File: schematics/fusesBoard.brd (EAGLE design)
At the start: 25 parts, among them Q1 IRF540, Q2 IRF540, Q3 IRF540

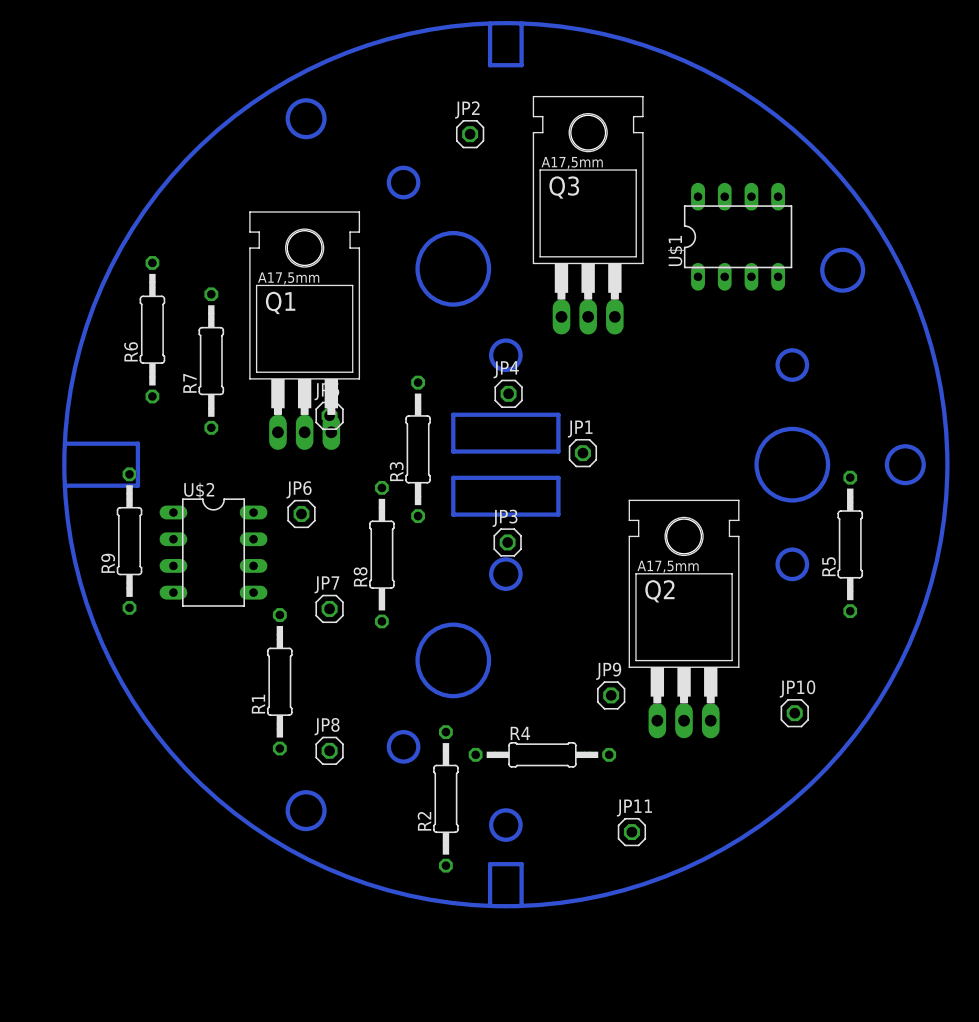
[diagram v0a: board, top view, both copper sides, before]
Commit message: разведена плата для пережигателей
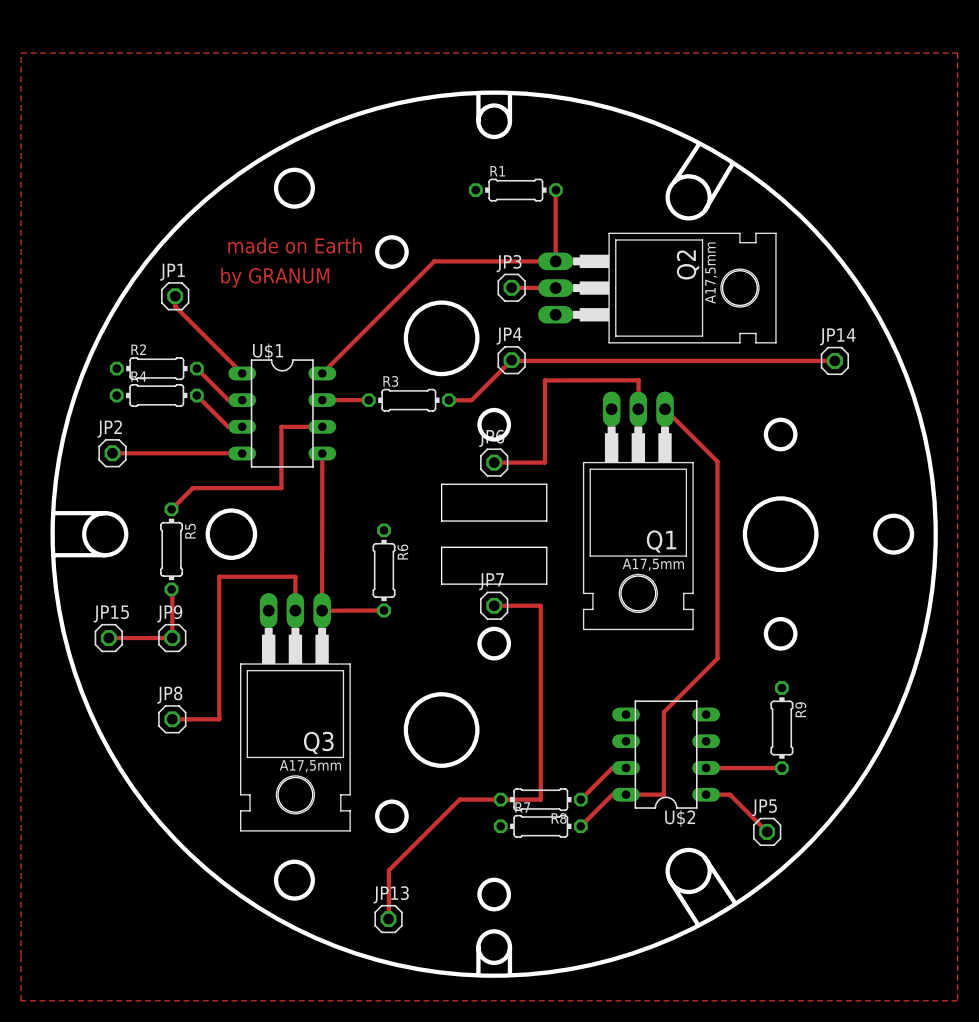
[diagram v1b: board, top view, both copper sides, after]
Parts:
- removed JP10, JP11: (no value), pinhead:1X01
- added JP13, JP14, JP15: (no value), pinhead:1X01
- R1: value (none) -> 10k; device rcl:0207/12 -> resistor:0204/7
- R2, R7, R8: device rcl:0207/12 -> resistor:0204/7
- R3: value (none) -> 1k; device rcl:0207/12 -> resistor:0204/7
- R4: value 1k -> (none); device rcl:0207/12 -> resistor:0204/7
- R5: value 10k -> 1k; device rcl:0207/12 -> resistor:0204/7
- R6: value 1k -> 10k; device rcl:0207/12 -> resistor:0204/7
- R9: value 10k -> (none); device rcl:0207/12 -> resistor:0204/7
- moved R5 64.6 mm to (14.3, 38.7), turned to 270 degrees
- moved R9 64.6 mm to (72.4, 21.7), turned to 270 degrees
- moved JP5 57.4 mm to (71.0, 11.8)
- moved R7 54.2 mm to (49.4, 12.3), turned to 0 degrees
- moved R1 51.9 mm to (47.1, 72.8), turned to 0 degrees
- moved R4 50.1 mm to (12.9, 53.3)
- moved R2 49.3 mm to (12.9, 55.9), turned to 0 degrees
- moved Q3 49.3 mm to (26.1, 26.5), turned to 180 degrees
- moved U$2 47.1 mm to (61.4, 19.1), turned to 90 degrees
- moved U$1 46.5 mm to (24.9, 51.6), turned to 270 degrees
- moved JP2 45.6 mm to (8.70, 47.8)
- moved JP9 42.1 mm to (14.4, 30.2)
- moved JP1 41.6 mm to (14.7, 62.7)
- moved Q2 35.3 mm to (57.2, 63.5), turned to 270 degrees
- moved Q1 33.4 mm to (58.7, 45.6), turned to 180 degrees
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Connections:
- removed net +7V: JP4.1, JP7.1, JP9.1, R4.2, R6.2, R8.1
- new net VCC1: JP13.1, JP7.1, R8.2
- new net VCC2: JP14.1, JP4.1, R3.2
- new net VCC3: JP15.1, JP9.1, R5.2
- net GND: now also R4.1, R6.1; no longer R3.2, R5.1
- net N$10: now also R1.2; no longer R5.2
- net N$11: now also R3.1; no longer R4.1
- net N$15: now also R8.1; no longer R6.1
- net N$18: now also R9.2; no longer R1.2
- net N$20: now also R6.2; no longer R9.2
- net N$22: now also R5.1; no longer R8.2
- net N$26: now also R4.2; no longer R3.1
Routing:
- net N$12: track 0.00 -> 50.0 mm
- net VCC1: track 0.00 -> 44.8 mm
- net VCC2: track 0.00 -> 38.4 mm
- net N$10: track 0.00 -> 33.4 mm
- net N$23: track 0.00 -> 28.5 mm
- net N$1: track 0.00 -> 24.3 mm
- net N$7: track 21.8 -> 0.00 mm
- net N$22: track 0.00 -> 21.0 mm
- net N$20: track 0.00 -> 20.8 mm
- net N$9: track 13.9 -> 0.00 mm
- net N$5: track 13.5 -> 0.00 mm
- net N$2 (its old number): track 13.5 -> 0.00 mm
- net N$25: track 0.00 -> 12.4 mm
- net VCC3: track 0.00 -> 10.7 mm
- net N$4: track 10.0 -> 0.00 mm
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- added copper zone on layer 1, net GND
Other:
- board outline added: 84 x 84 mm
- board text added: "by GRANUM"
- board text added: "made on Earth"
